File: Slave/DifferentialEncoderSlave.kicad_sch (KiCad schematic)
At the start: 32 parts, among them J2 Debug, J3 Thermistor, U1 ADM4852, U2 STM32G4A1KEU4, U3 LP5907MFX-3.3, U4 MA730

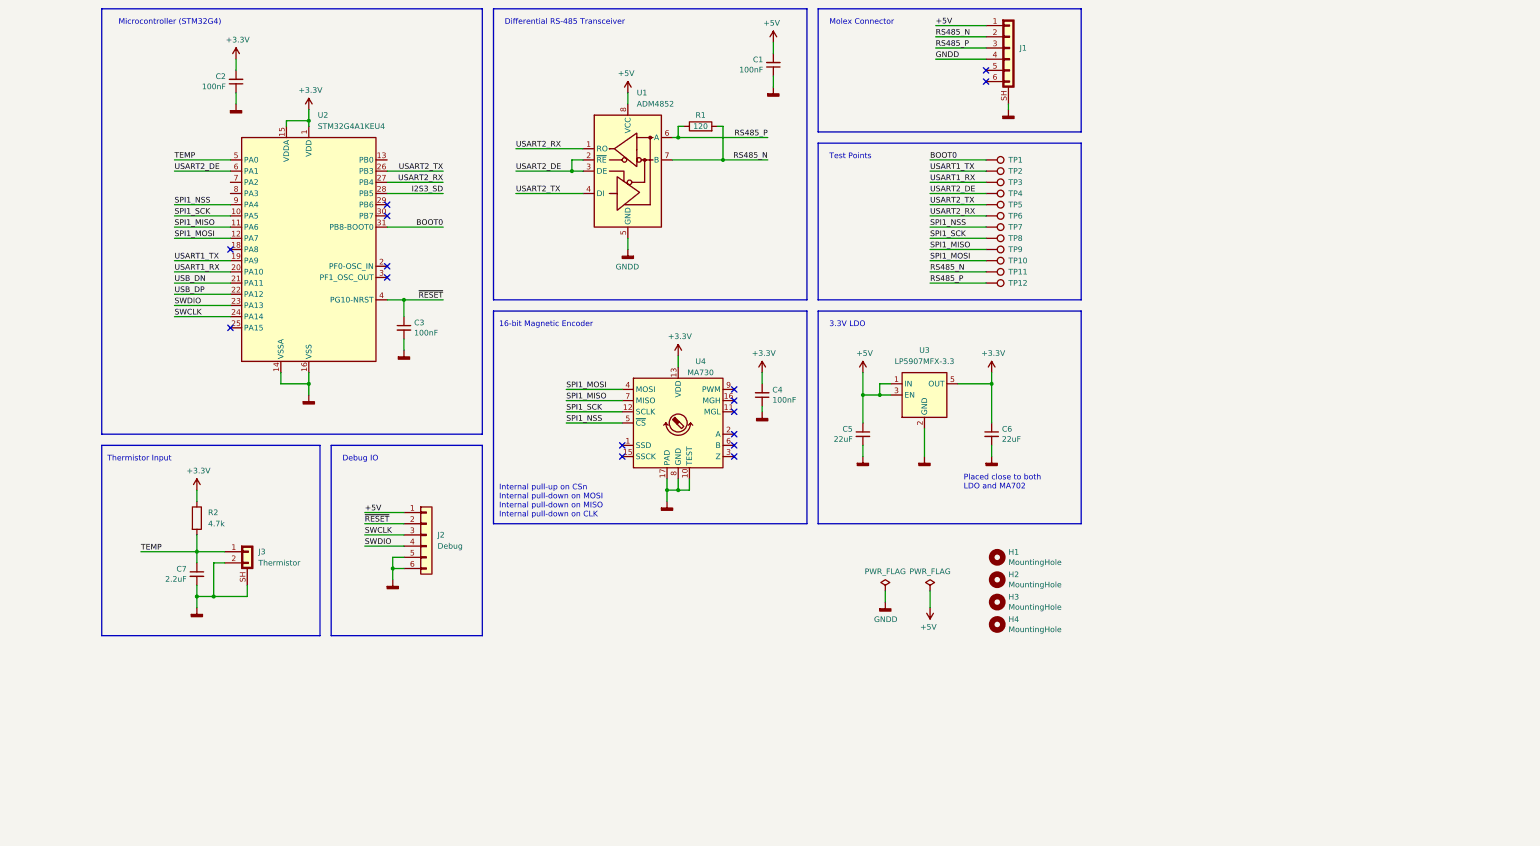
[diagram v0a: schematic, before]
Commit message: Solomon redux
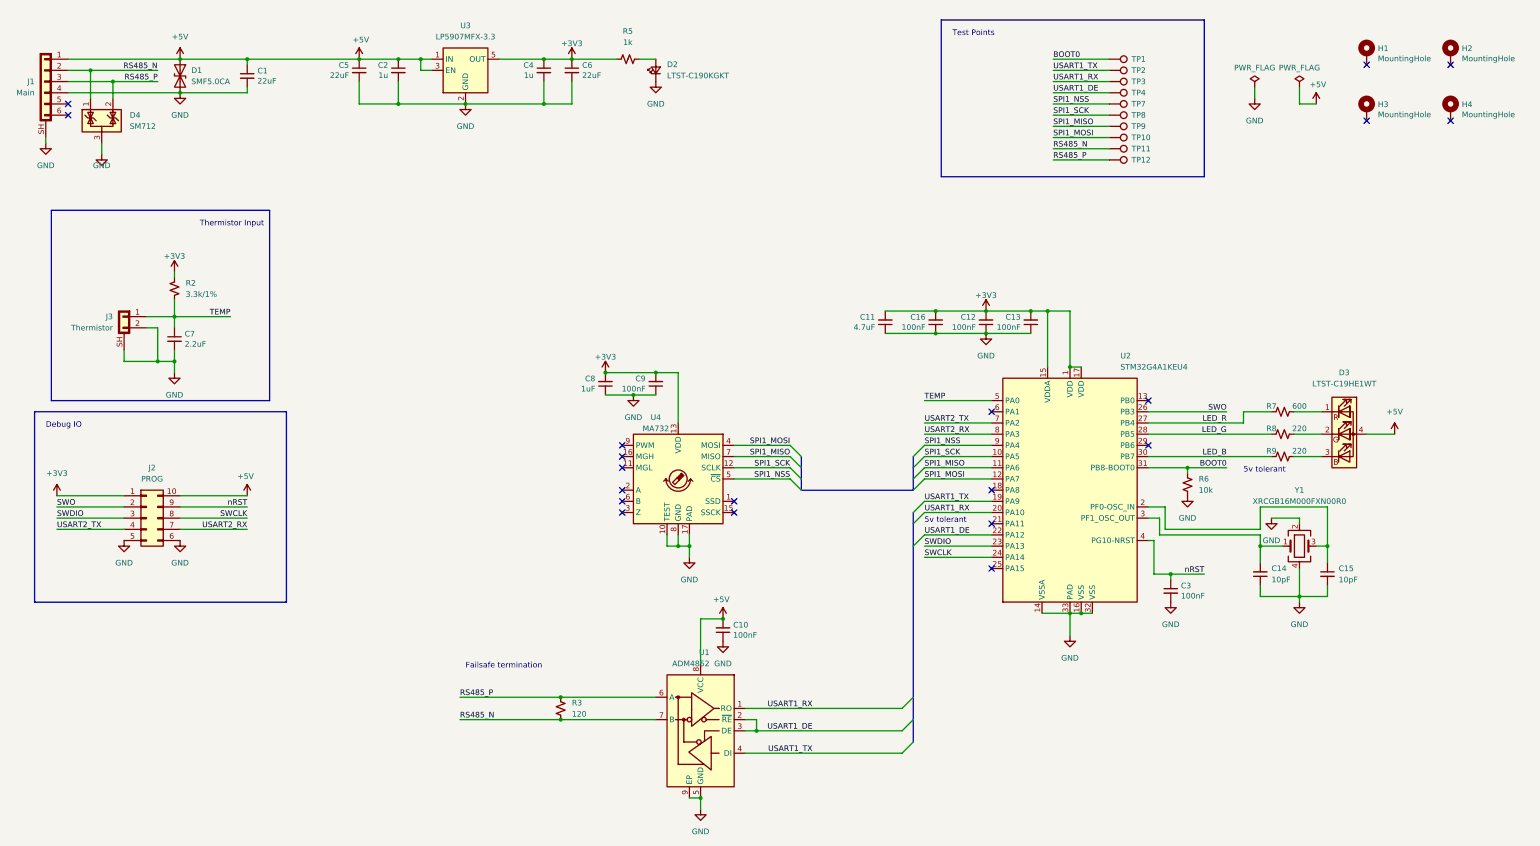
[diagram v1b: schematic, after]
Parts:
- removed J2: Debug, Connector:Tag-Connect_TC2030-IDC-NL_2x03_P1.27mm_Vertical, symbol Connector_Generic:Conn_01x06
- removed R1: 120, Resistor_SMD:R_0402_1005Metric, symbol Device:R
- removed TP5, TP6: TestPoint, ODrive_KiCad:TestPoint_Pad_D1.0mm, symbol Connector:TestPoint
- added C10, C12, C13, C16, C9: 100nF, Capacitor_SMD:C_0402_1005Metric, symbol Device:C_Small
- added C11: 4.7uF, Capacitor_SMD:C_0603_1608Metric, symbol Device:C_Small
- added C14, C15: 10pF, Capacitor_SMD:C_0402_1005Metric, symbol Device:C_Small
- added C8: 1uF, Capacitor_SMD:C_0402_1005Metric, symbol Device:C_Small
- added D1: SMF5.0CA, Diode_SMD:D_SOD-123F, symbol Device:D_TVS
- added D2: LTST-C190KGKT, LED_SMD:LED_0603_1608Metric, symbol Device:LED_Small
- added D3: LTST-C19HE1WT, LED_SMD:LED_LiteOn_LTST-C19HE1WT, symbol Device:LED_RGBA
- added D4: SM712, Package_TO_SOT_SMD:SOT-23, symbol Power_Protection:NUP2105L
- added J2: PROG, Connector:Tag-Connect_TC2050-IDC-NL_2x05_P1.27mm_Vertical_with_bottom_clip, symbol Connector_Generic:Conn_02x05_Counter_Clockwise
- added R3: 120, Resistor_SMD:R_0805_2012Metric, symbol Device:R_Small_US
- added R5: 1k, Resistor_SMD:R_0402_1005Metric, symbol Device:R_Small_US
- added R6: 10k, Resistor_SMD:R_0402_1005Metric, symbol Device:R_Small_US
- added R7: 600, Resistor_SMD:R_0402_1005Metric, symbol Device:R_Small_US
- added R8, R9: 220, Resistor_SMD:R_0402_1005Metric, symbol Device:R_Small_US
- added Y1: XRCGB16M000FXN00R0, Crystal:Crystal_SMD_2016-4Pin_2.0x1.6mm, symbol Device:Crystal_GND24
- C1: value 100nF -> 22uF; footprint Capacitor_SMD:C_0402_1005Metric -> Capacitor_SMD:C_0805_2012Metric
- C2, C4: value 100nF -> 1u
- H1, H2, H3, H4: footprint MountingHole:MountingHole_3mm -> mag-encoder:MountingHole_3.1mm_Pad_Via; symbol Mechanical:MountingHole -> Mechanical:MountingHole_Pad
- J1: value (none) -> Main; footprint (none) -> Connector_Molex:Molex_CLIK-Mate_502585-0670_1x06-1MP_P1.50mm_Horizontal
- R2: value 4.7k -> 3.3k/1%; symbol Device:R -> Device:R_Small_US
- TP1, TP10, TP11, TP12, TP2, TP3, TP4, TP7, TP8, TP9: footprint ODrive_KiCad:TestPoint_Pad_D1.0mm -> TestPoint:TestPoint_Pad_1.0x1.0mm
- U4: value MA730 -> MA732
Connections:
- net USB_DP is gone; now on net USART1_DE: U2.22 (PA12)
- net +3V3: now also C4.1, C11.2, C12.2, C13.2, C16.2, C8.2, C9.2, J2.1 (Pin_1), R5.1; no longer C2.2, C4.2
- net +5V: now also C1.1, C2.1, C10.2, D1.1 (A1), D3.4 (A), J2.10 (Pin_10); no longer C1.2
- net BOOT0: now also R6.1
- net RS485_N: now also D4.1 (K), R3.2
- net RS485_P: now also D4.2 (K), R3.1
- net SWCLK: now also J2.8 (Pin_8)
- net SWDIO: now also J2.3 (Pin_3)
- net USART1_RX: now also U1.1 (RO)
- net USART1_TX: now also U1.4 (DI)
- net USART2_RX: now also U2.8 (PA3), J2.7 (Pin_7); no longer U1.1 (RO), U2.27 (PB4)
- net USART2_TX: now also U2.7 (PA2), J2.4 (Pin_4); no longer U1.4 (DI), U2.26 (PB3)
- net at U2.2 (PF0-OSC_IN): now also C15.1, Y1.3
- net at U2.3 (PF1_OSC_OUT): now also C14.2, Y1.1
- net LED_B: now reaches U2.30 (PB7)
- net LED_B: now also R9.1
- net GNDD renamed GND
- net GND: now also C1.2, C2.2, C4.2, U1.9 (EP), C10.1, C11.1, C12.1, C13.1, C14.1, C15.2, C16.1, C8.1, C9.1, D1.2 (A2), D2.1 (K), D4.3 (A), J2.5 (Pin_5), J2.6 (Pin_6), R6.2, Y1.2, Y1.4; no longer C1.1, C2.1, C4.1, U1.PAD
- net I2S3_SD renamed LED_G
- net LED_G: now also R8.1
- net USART2_DE renamed USART1_DE
- net USART1_DE: no longer U2.6 (PA1)
- net USB_DN: no longer names the net of U2.21 (PA11)
- net ~{RESET} renamed nRST
- net nRST: now also J2.9 (Pin_9)
- new net: D2.2 (A), R5.2
- new net: D3.1 (RK), R7.2
- new net: D3.2 (GK), R8.2
- new net: D3.3 (BK), R9.2
- new net LED_R: R7.1, U2.27 (PB4)
- new net SWO: J2.2 (Pin_2), U2.26 (PB3)
- no-connect marks 16 -> 20
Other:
- note added: "5v tolerant"
- note added: "Failsafe termination"
- note removed: "16-bit Magnetic Encoder"
- note removed: "3.3V LDO"
- note removed: "Differential RS-485 Transceiver"
- note removed: "Internal pull-up on CSn Internal pull-down on MOSI Internal pull-down on MISO Internal pull-down on CLK"
- note removed: "Microcontroller (STM32G4)"
- note removed: "Molex Connector"
- note removed: "Placed close to both LDO and MA702"
- moved on the sheet: C3, C5, C6, C7, J3, TP1, TP10, TP11, TP12, TP2, TP3, TP4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
